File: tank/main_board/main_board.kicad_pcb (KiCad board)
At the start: 2 copper layers, 66.5 x 56.2 mm, 41 parts, among them J1 PowerOut, J10 PowerMotor, J11 SigOut, J12 Spk, J14 M0, J15 M1, J16 M2, J2 PowerIn, J3 Encoder0, J4 Encoder1, J5 Encoder2, J6 Encoder3, J7 Bump0, J8 Bump1, J9 Programming Header, U1 L7805, U4 L293D, U5 L293D, Y1 Crystal

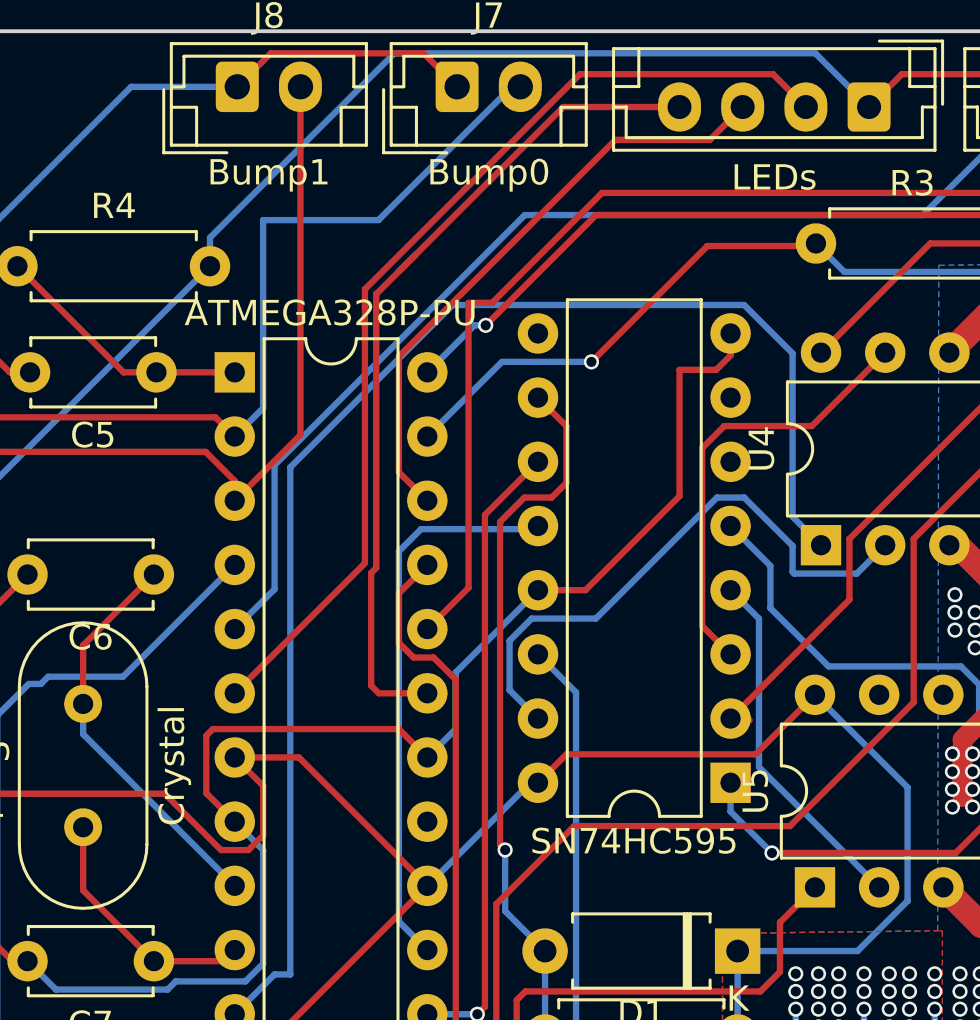
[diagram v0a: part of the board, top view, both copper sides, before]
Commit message: fixes
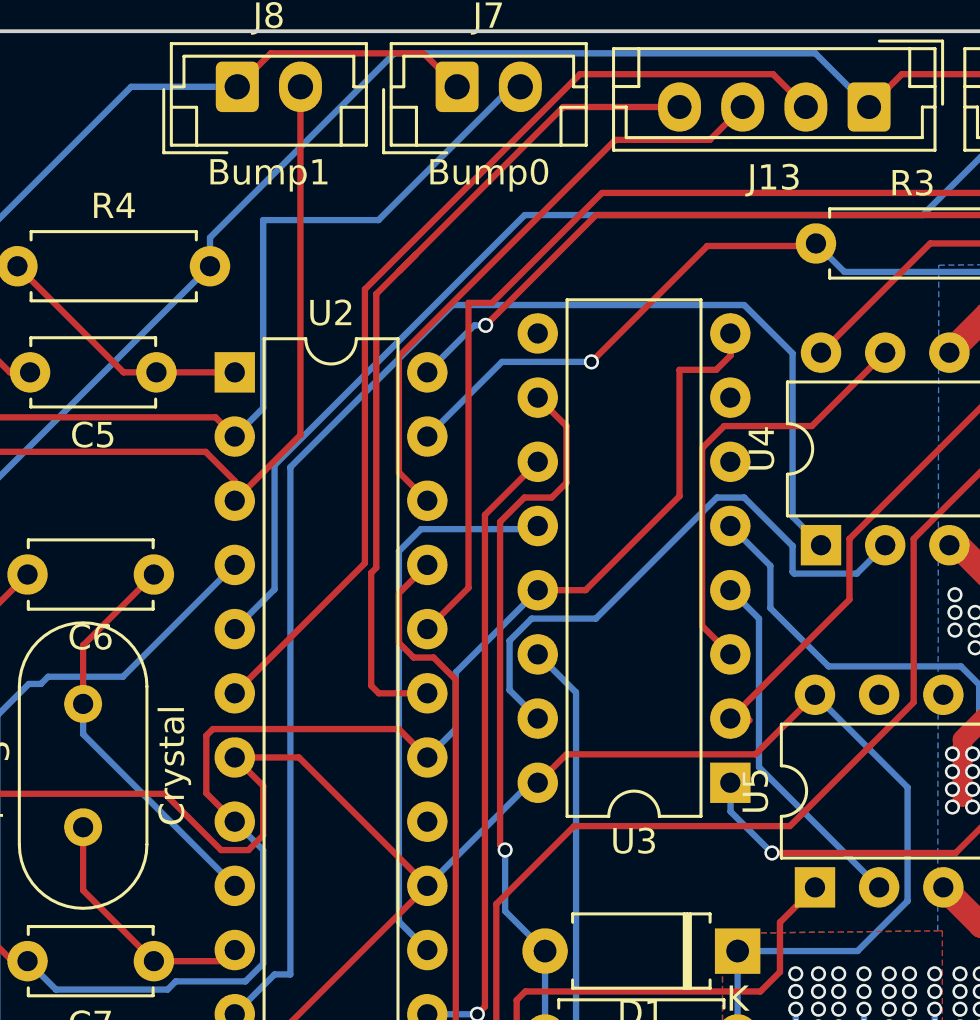
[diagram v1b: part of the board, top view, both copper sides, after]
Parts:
- removed SN74HC595: SN74HC595, custom:DIP-16_W7.62mm
- added U3: SN74HC595, custom:DIP-16_W7.62mm, F.Cu at (133.6, 103.2)
- renumbered LEDs to J13, ATMEGA328P-PU to U2
